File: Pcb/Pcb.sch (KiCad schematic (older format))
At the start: 123 parts, among them J1 TRRS, Q1 2N7002, SW1 SW_Push, SW10 SW_Push, SW11 SW_Push, SW12 SW_Push, SW13 SW_Push, SW14 SW_Push, SW15 SW_Push, SW16 SW_Push, SW17 SW_Push, SW18 SW_Push, SW19 SW_Push, SW2 SW2, SW20 SW_Push, SW21 SW_Push, SW22 SW_Push, SW23 SW_Push, SW24 SW_Push, SW25 SW_Push, SW26 SW_Push, SW27 SW_Push, SW28 SW_Push, SW29 SW_Push, SW3 SW_Push, SW4 SW_Push, SW5 SW_Push, SW6 SW_Push, SW7 SW_Push, SW8 SW_Push, SW9 SW_Push, U1 ProMicro

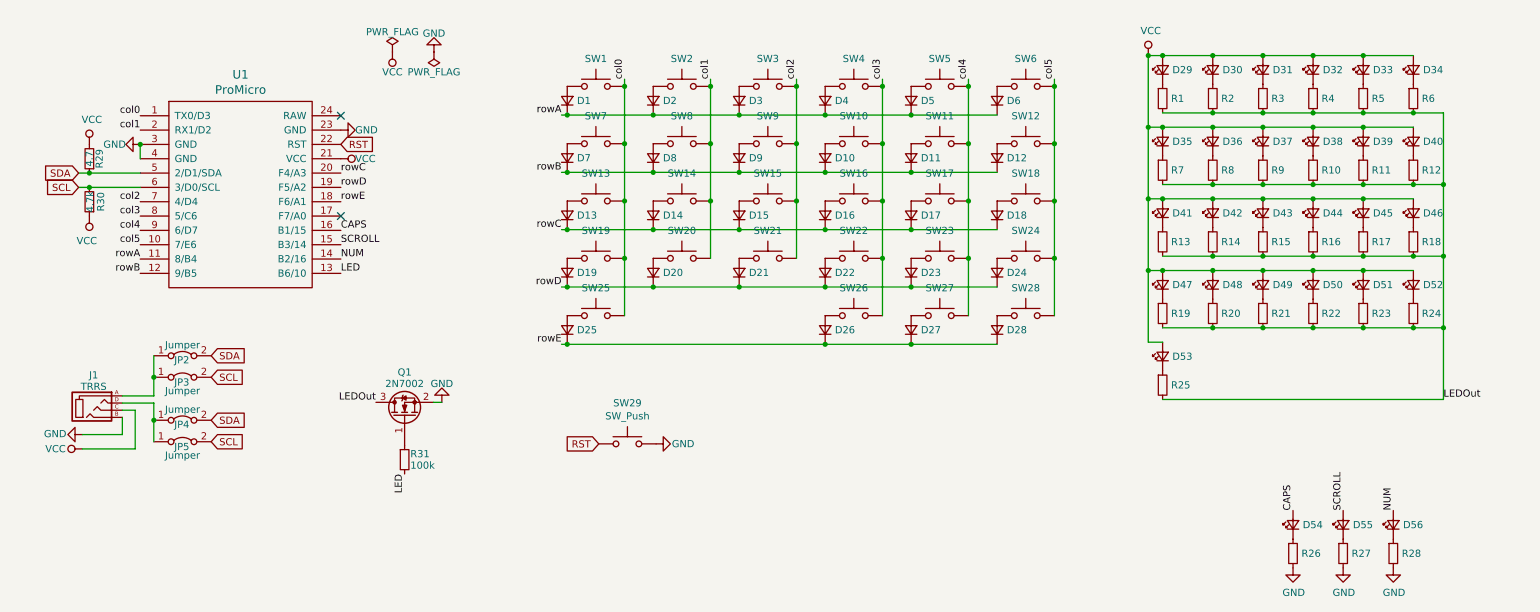
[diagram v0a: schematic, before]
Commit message: Updated footprints
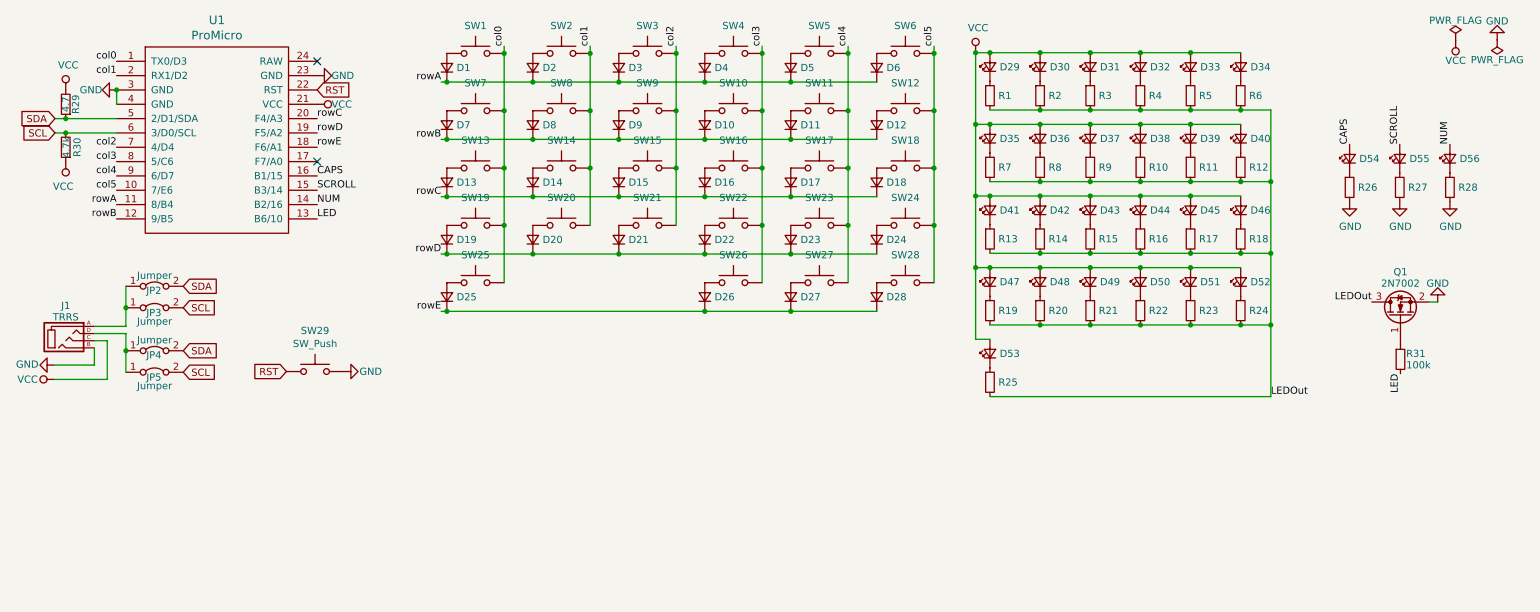
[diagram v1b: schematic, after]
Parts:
- J1: footprint Used_Footprints:TRRS_2Side -> 1symblos:MJ-4PP-9_Dual
- JP2, JP3, JP4, JP5: footprint (none) -> 1kbd:jumper
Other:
- moved on the sheet: D1, D10, D11, D12, D13, D14, D15, D16, D17, D18, D19, D2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

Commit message: Updated footprints
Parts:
- SW1, SW10, SW11, SW12, SW13, SW14, SW15, SW16, SW17, SW18, SW19, SW2, SW20, SW21, SW22, SW23, SW24, SW25, SW26, SW27, SW28, SW3, SW4, SW5, SW6, SW7, SW8, SW9: footprint Used_Footprints:MX_Two_Side -> 1symblos:cherry
- SW29: footprint Used_Footprints:MX_Two_Side -> Used_Footprints:Reset_Switch
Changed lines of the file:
@@
 F 0 "SW1" H 3745 1083 50  0000 C CNN
 F 1 "SW_Push" H 3745 1084 50  0001 C CNN
-F 2 "Used_Footprints:MX_Two_Side" H 3745 1090 50  0001 C CNN
+F 2 "1symblos:cherry" H 3745 1090 50  0001 C CNN
 F 3 "~" H 3745 1090 50  0001 C CNN
 	1    3745 890
@@
 F 0 "SW2" H 4345 1083 50  0000 C CNN
 F 1 "SW2" H 4345 1084 50  0001 C CNN
-F 2 "Used_Footprints:MX_Two_Side" H 4345 1090 50  0001 C CNN
+F 2 "1symblos:cherry" H 4345 1090 50  0001 C CNN
 F 3 "~" H 4345 1090 50  0001 C CNN
 	1    4345 890
@@
 F 0 "SW3" H 4945 1083 50  0000 C CNN
 F 1 "SW_Push" H 4945 1084 50  0001 C CNN
-F 2 "Used_Footprints:MX_Two_Side" H 4945 1090 50  0001 C CNN
+F 2 "1symblos:cherry" H 4945 1090 50  0001 C CNN
 F 3 "~" H 4945 1090 50  0001 C CNN
 	1    4945 890
@@
 F 0 "SW4" H 5545 1083 50  0000 C CNN
 F 1 "SW_Push" H 5545 1084 50  0001 C CNN
-F 2 "Used_Footprints:MX_Two_Side" H 5545 1090 50  0001 C CNN
+F 2 "1symblos:cherry" H 5545 1090 50  0001 C CNN
 F 3 "~" H 5545 1090 50  0001 C CNN
 	1    5545 890
@@
 F 0 "SW5" H 6145 1083 50  0000 C CNN
 F 1 "SW_Push" H 6145 1084 50  0001 C CNN
-F 2 "Used_Footprints:MX_Two_Side" H 6145 1090 50  0001 C CNN
+F 2 "1symblos:cherry" H 6145 1090 50  0001 C CNN
 F 3 "~" H 6145 1090 50  0001 C CNN
 	1    6145 890
@@
 F 0 "SW6" H 6745 1083 50  0000 C CNN
 F 1 "SW_Push" H 6745 1084 50  0001 C CNN
-F 2 "Used_Footprints:MX_Two_Side" H 6745 1090 50  0001 C CNN
+F 2 "1symblos:cherry" H 6745 1090 50  0001 C CNN
 F 3 "~" H 6745 1090 50  0001 C CNN
 	1    6745 890
@@
 F 0 "SW7" H 3745 1483 50  0000 C CNN
 F 1 "SW_Push" H 3745 1484 50  0001 C CNN
-F 2 "Used_Footprints:MX_Two_Side" H 3745 1490 50  0001 C CNN
+F 2 "1symblos:cherry" H 3745 1490 50  0001 C CNN
 F 3 "~" H 3745 1490 50  0001 C CNN
 	1    3745 1290
@@
 F 0 "SW8" H 4345 1483 50  0000 C CNN
 F 1 "SW_Push" H 4345 1484 50  0001 C CNN
-F 2 "Used_Footprints:MX_Two_Side" H 4345 1490 50  0001 C CNN
+F 2 "1symblos:cherry" H 4345 1490 50  0001 C CNN
 F 3 "~" H 4345 1490 50  0001 C CNN
 	1    4345 1290
@@
 F 0 "SW9" H 4945 1483 50  0000 C CNN
 F 1 "SW_Push" H 4945 1484 50  0001 C CNN
-F 2 "Used_Footprints:MX_Two_Side" H 4945 1490 50  0001 C CNN
+F 2 "1symblos:cherry" H 4945 1490 50  0001 C CNN
 F 3 "~" H 4945 1490 50  0001 C CNN
 	1    4945 1290
@@
 F 0 "SW10" H 5545 1483 50  0000 C CNN
 F 1 "SW_Push" H 5545 1484 50  0001 C CNN
-F 2 "Used_Footprints:MX_Two_Side" H 5545 1490 50  0001 C CNN
+F 2 "1symblos:cherry" H 5545 1490 50  0001 C CNN
 F 3 "~" H 5545 1490 50  0001 C CNN
 	1    5545 1290
@@
 F 0 "SW11" H 6145 1483 50  0000 C CNN
 F 1 "SW_Push" H 6145 1484 50  0001 C CNN
-F 2 "Used_Footprints:MX_Two_Side" H 6145 1490 50  0001 C CNN
+F 2 "1symblos:cherry" H 6145 1490 50  0001 C CNN
 F 3 "~" H 6145 1490 50  0001 C CNN
 	1    6145 1290
@@
 F 0 "SW12" H 6745 1483 50  0000 C CNN
 F 1 "SW_Push" H 6745 1484 50  0001 C CNN
-F 2 "Used_Footprints:MX_Two_Side" H 6745 1490 50  0001 C CNN
+F 2 "1symblos:cherry" H 6745 1490 50  0001 C CNN
 F 3 "~" H 6745 1490 50  0001 C CNN
 	1    6745 1290
@@
 F 0 "SW13" H 3745 1883 50  0000 C CNN
 F 1 "SW_Push" H 3745 1884 50  0001 C CNN
-F 2 "Used_Footprints:MX_Two_Side" H 3745 1890 50  0001 C CNN
+F 2 "1symblos:cherry" H 3745 1890 50  0001 C CNN
 F 3 "~" H 3745 1890 50  0001 C CNN
 	1    3745 1690
@@
 F 0 "SW14" H 4345 1883 50  0000 C CNN
 F 1 "SW_Push" H 4345 1884 50  0001 C CNN
-F 2 "Used_Footprints:MX_Two_Side" H 4345 1890 50  0001 C CNN
+F 2 "1symblos:cherry" H 4345 1890 50  0001 C CNN
 F 3 "~" H 4345 1890 50  0001 C CNN
 	1    4345 1690
@@
 F 0 "SW15" H 4945 1883 50  0000 C CNN
 F 1 "SW_Push" H 4945 1884 50  0001 C CNN
-F 2 "Used_Footprints:MX_Two_Side" H 4945 1890 50  0001 C CNN
+F 2 "1symblos:cherry" H 4945 1890 50  0001 C CNN
 F 3 "~" H 4945 1890 50  0001 C CNN
 	1    4945 1690
@@
 F 0 "SW16" H 5545 1883 50  0000 C CNN
 F 1 "SW_Push" H 5545 1884 50  0001 C CNN
-F 2 "Used_Footprints:MX_Two_Side" H 5545 1890 50  0001 C CNN
+F 2 "1symblos:cherry" H 5545 1890 50  0001 C CNN
 F 3 "~" H 5545 1890 50  0001 C CNN
 	1    5545 1690
@@
 F 0 "SW17" H 6145 1883 50  0000 C CNN
 F 1 "SW_Push" H 6145 1884 50  0001 C CNN
-F 2 "Used_Footprints:MX_Two_Side" H 6145 1890 50  0001 C CNN
+F 2 "1symblos:cherry" H 6145 1890 50  0001 C CNN
 F 3 "~" H 6145 1890 50  0001 C CNN
 	1    6145 1690
@@
 F 0 "SW18" H 6745 1883 50  0000 C CNN
 F 1 "SW_Push" H 6745 1884 50  0001 C CNN
-F 2 "Used_Footprints:MX_Two_Side" H 6745 1890 50  0001 C CNN
+F 2 "1symblos:cherry" H 6745 1890 50  0001 C CNN
 F 3 "~" H 6745 1890 50  0001 C CNN
 	1    6745 1690
@@
 F 0 "SW19" H 3745 2283 50  0000 C CNN
 F 1 "SW_Push" H 3745 2284 50  0001 C CNN
-F 2 "Used_Footprints:MX_Two_Side" H 3745 2290 50  0001 C CNN
+F 2 "1symblos:cherry" H 3745 2290 50  0001 C CNN
 F 3 "~" H 3745 2290 50  0001 C CNN
 	1    3745 2090
@@
 F 0 "SW20" H 4345 2283 50  0000 C CNN
 F 1 "SW_Push" H 4345 2284 50  0001 C CNN
-F 2 "Used_Footprints:MX_Two_Side" H 4345 2290 50  0001 C CNN
+F 2 "1symblos:cherry" H 4345 2290 50  0001 C CNN
 F 3 "~" H 4345 2290 50  0001 C CNN
 	1    4345 2090
@@
 F 0 "SW21" H 4945 2283 50  0000 C CNN
 F 1 "SW_Push" H 4945 2284 50  0001 C CNN
-F 2 "Used_Footprints:MX_Two_Side" H 4945 2290 50  0001 C CNN
+F 2 "1symblos:cherry" H 4945 2290 50  0001 C CNN
 F 3 "~" H 4945 2290 50  0001 C CNN
 	1    4945 2090
@@
 F 0 "SW22" H 5545 2283 50  0000 C CNN
 F 1 "SW_Push" H 5545 2284 50  0001 C CNN
-F 2 "Used_Footprints:MX_Two_Side" H 5545 2290 50  0001 C CNN
+F 2 "1symblos:cherry" H 5545 2290 50  0001 C CNN
 F 3 "~" H 5545 2290 50  0001 C CNN
 	1    5545 2090
@@
 F 0 "SW23" H 6145 2283 50  0000 C CNN
 F 1 "SW_Push" H 6145 2284 50  0001 C CNN
-F 2 "Used_Footprints:MX_Two_Side" H 6145 2290 50  0001 C CNN
+F 2 "1symblos:cherry" H 6145 2290 50  0001 C CNN
 F 3 "~" H 6145 2290 50  0001 C CNN
 	1    6145 2090
@@
 F 0 "SW24" H 6745 2283 50  0000 C CNN
 F 1 "SW_Push" H 6745 2284 50  0001 C CNN
-F 2 "Used_Footprints:MX_Two_Side" H 6745 2290 50  0001 C CNN
+F 2 "1symblos:cherry" H 6745 2290 50  0001 C CNN
 F 3 "~" H 6745 2290 50  0001 C CNN
 	1    6745 2090
@@
 F 0 "SW25" H 3745 2683 50  0000 C CNN
 F 1 "SW_Push" H 3745 2684 50  0001 C CNN
-F 2 "Used_Footprints:MX_Two_Side" H 3745 2690 50  0001 C CNN
+F 2 "1symblos:cherry" H 3745 2690 50  0001 C CNN
 F 3 "~" H 3745 2690 50  0001 C CNN
 	1    3745 2490
@@
 F 0 "SW26" H 5545 2683 50  0000 C CNN
 F 1 "SW_Push" H 5545 2684 50  0001 C CNN
-F 2 "Used_Footprints:MX_Two_Side" H 5545 2690 50  0001 C CNN
+F 2 "1symblos:cherry" H 5545 2690 50  0001 C CNN
 F 3 "~" H 5545 2690 50  0001 C CNN
 	1    5545 2490
@@
 F 0 "SW27" H 6145 2683 50  0000 C CNN
 F 1 "SW_Push" H 6145 2684 50  0001 C CNN
-F 2 "Used_Footprints:MX_Two_Side" H 6145 2690 50  0001 C CNN
+F 2 "1symblos:cherry" H 6145 2690 50  0001 C CNN
 F 3 "~" H 6145 2690 50  0001 C CNN
 	1    6145 2490
@@
 F 0 "SW28" H 6745 2683 50  0000 C CNN
 F 1 "SW_Push" H 6745 2684 50  0001 C CNN
-F 2 "Used_Footprints:MX_Two_Side" H 6745 2690 50  0001 C CNN
+F 2 "1symblos:cherry" H 6745 2690 50  0001 C CNN
 F 3 "~" H 6745 2690 50  0001 C CNN
 	1    6745 2490
@@
 F 0 "SW29" H 2625 3395 50  0000 C CNN
 F 1 "SW_Push" H 2625 3304 50  0000 C CNN
-F 2 "Used_Footprints:MX_Two_Side" H 2625 3310 50  0001 C CNN
+F 2 "Used_Footprints:Reset_Switch" H 2625 3310 50  0001 C CNN
 F 3 "~" H 2625 3310 50  0001 C CNN
 	1    2625 3110
